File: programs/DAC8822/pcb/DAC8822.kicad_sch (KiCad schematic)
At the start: 32 parts, among them J1 TFT ST7735, J2 Conn_01x04_Pin, J3 Conn_01x04_Pin, J4 Screw_Terminal_01x02, J5 Conn_01x04_Pin, J6 Conn_01x04_Pin, U1 8BVG4, U10 TL431LP, U2 8BVG4, U3 RP2350B-WeAct, U4 OPA2277, U5 OPA2277, U6 OPA2277, U7 OPA2277, U8 LM7805

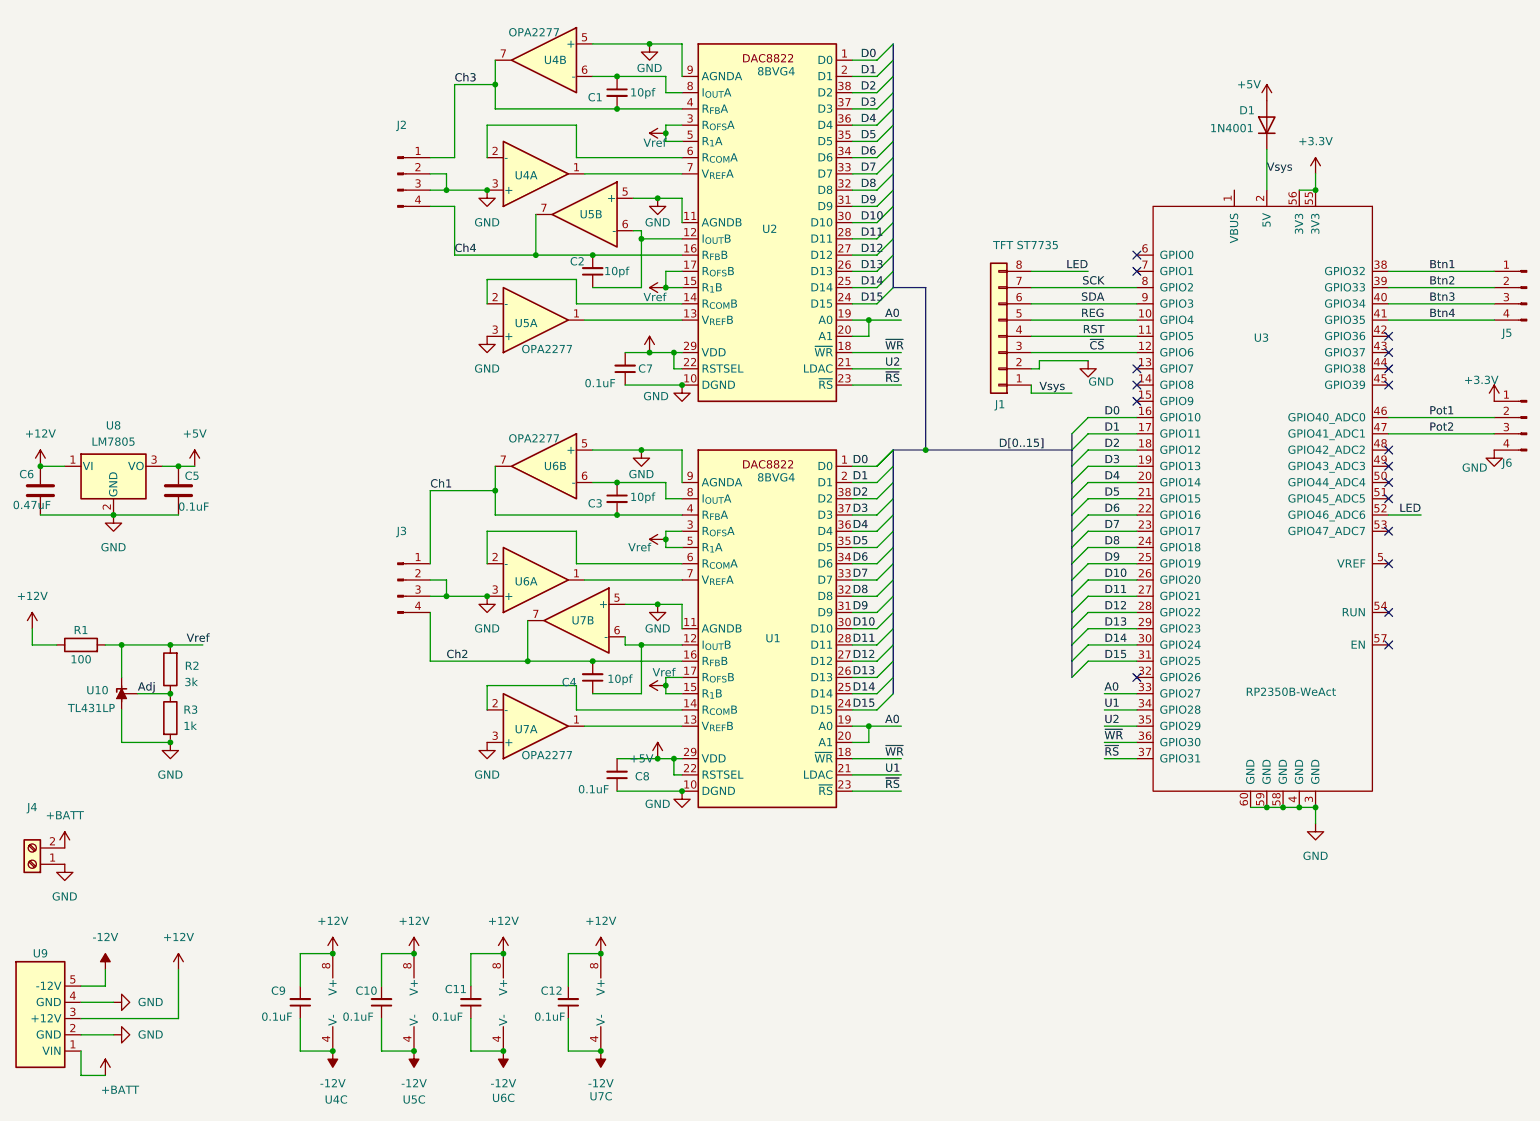
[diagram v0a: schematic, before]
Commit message: Add files via upload
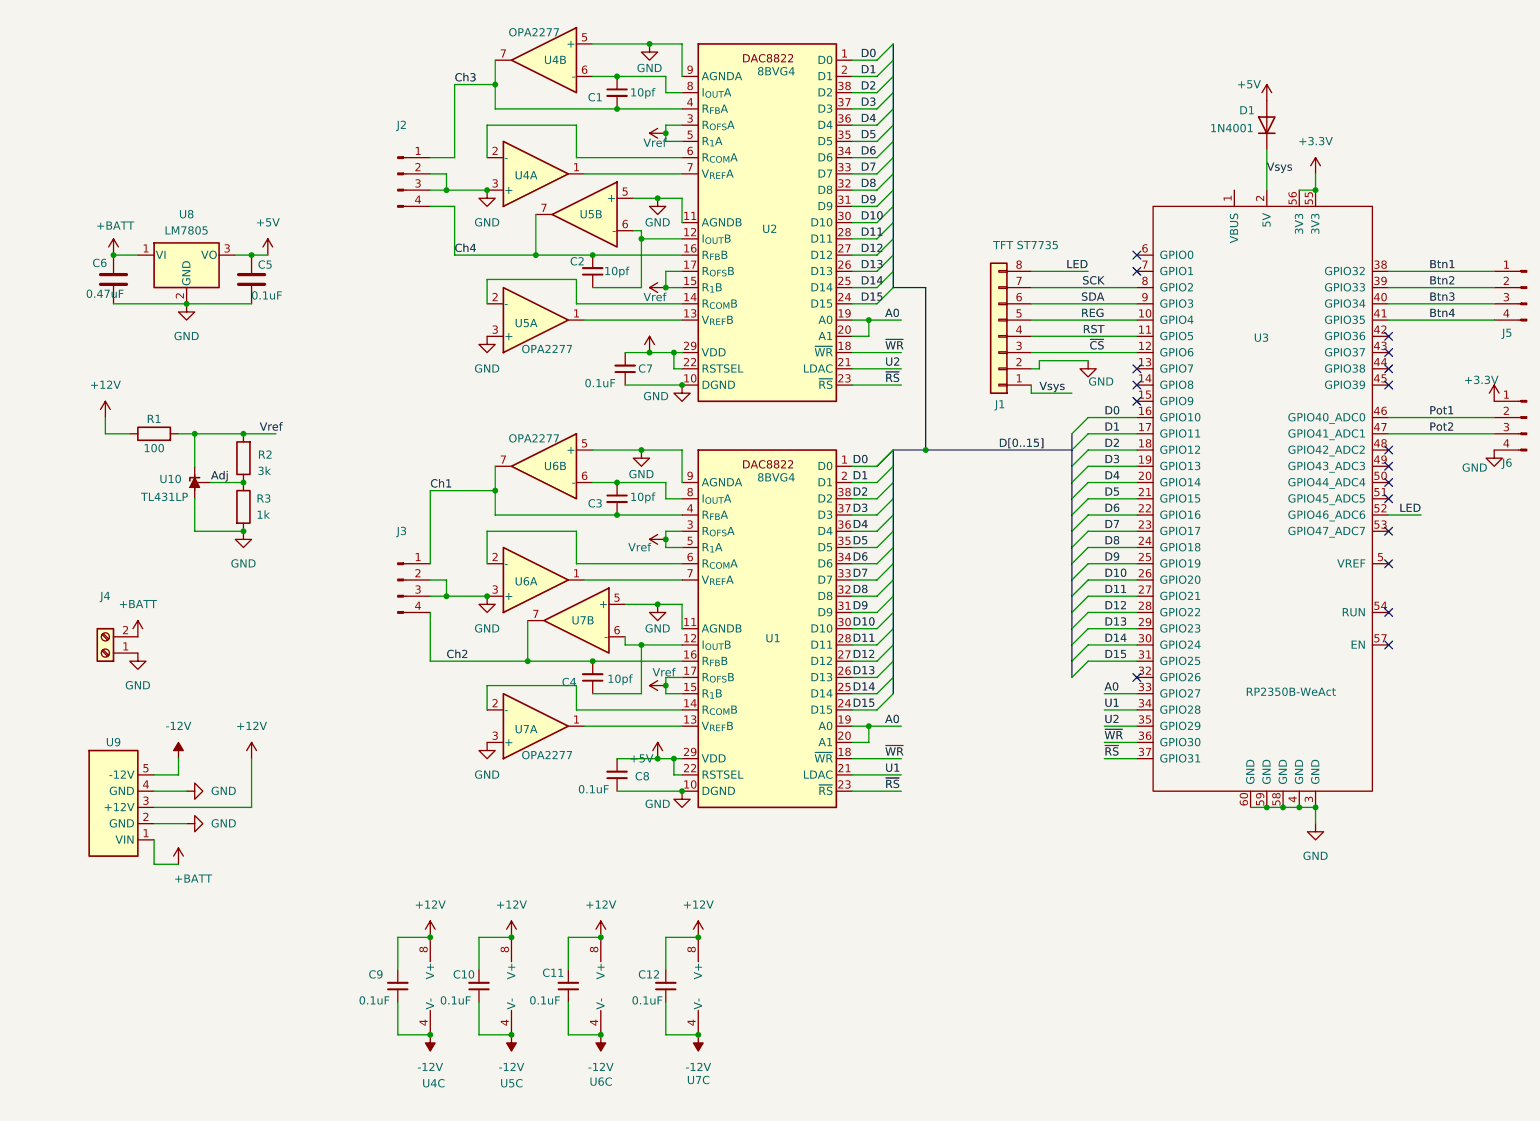
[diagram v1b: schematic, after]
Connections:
- net +12V: no longer C6.1, U8.1 (VI)
- net +BATT: now also C6.1, U8.1 (VI)
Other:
- title: 4 Ch Signal Generato Pico 2350 and DAC8822 x 2 -> 4 Ch Signal Generator Pico 2350 and DAC8822 x 2
- moved on the sheet: C10, C11, C12, C5, C6, C9, J4, R1, R2, R3, U10, U4C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

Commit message: Add files via upload
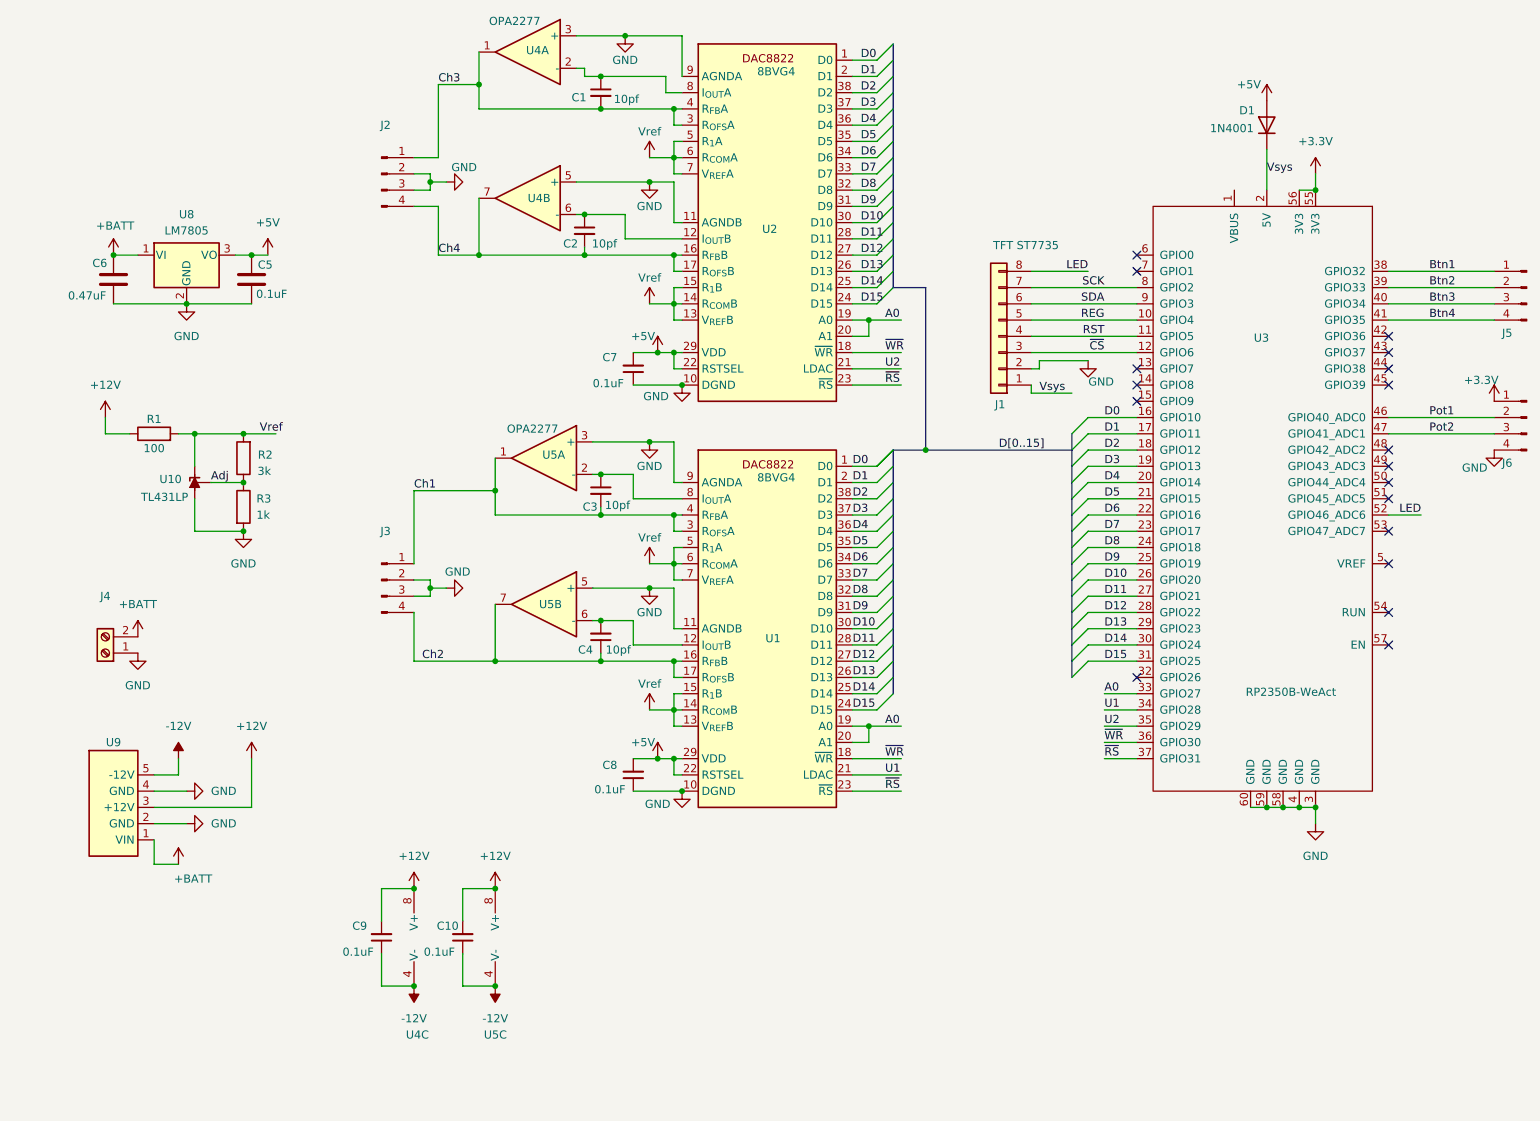
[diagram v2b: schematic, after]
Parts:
- removed C11, C12: 0.1uF, Capacitor_SMD:C_0805_2012Metric, symbol Device:C_Small
- removed U6, U7: OPA2277, Package_SO:SOIC-8_3.9x4.9mm_P1.27mm, symbol Amplifier_Operational:OPA2277
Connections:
- net Ch1: now also U1.3 (R_{OFS}A), U5.1
- net Ch2: now also C4.1, U1.17 (R_{OFS}B), U5.7; no longer C4.2
- net Ch3: now also U2.3 (R_{OFS}A), U4.1; no longer U4.7
- net Ch4: now also U2.17 (R_{OFS}B), U4.7; no longer U5.7
- net Vref: now also U1.13 (V_{REF}B), U1.14 (R_{COM}B), U1.6 (R_{COM}A), U1.7 (V_{REF}A), U2.13 (V_{REF}B), U2.14 (R_{COM}B), U2.6 (R_{COM}A), U2.7 (V_{REF}A); no longer U1.17 (R_{OFS}B), U1.3 (R_{OFS}A), U2.17 (R_{OFS}B), U2.3 (R_{OFS}A)
- net at C2.1, U2.12 (I_{OUT}B): now also U4.6 (-); no longer U5.6 (-)
- net at U5.2 (-): now also C3.1, U1.8 (I_{OUT}A); no longer U2.14 (R_{COM}B)
- net at U4.2 (-): now also C1.1, U2.8 (I_{OUT}A); no longer U2.6 (R_{COM}A)
- net at U1.12 (I_{OUT}B): now also C4.2, U5.6 (-); no longer C4.1
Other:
- moved on the sheet: C1, C10, C2, C4, C7, C8, C9, J2, J3, U4C, U5C
